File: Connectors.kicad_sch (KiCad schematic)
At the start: 13 parts, among them J5 Conn_02x03_Odd_Even, J6 Conn_02x03_Odd_Even, U12 TJA1051T/3

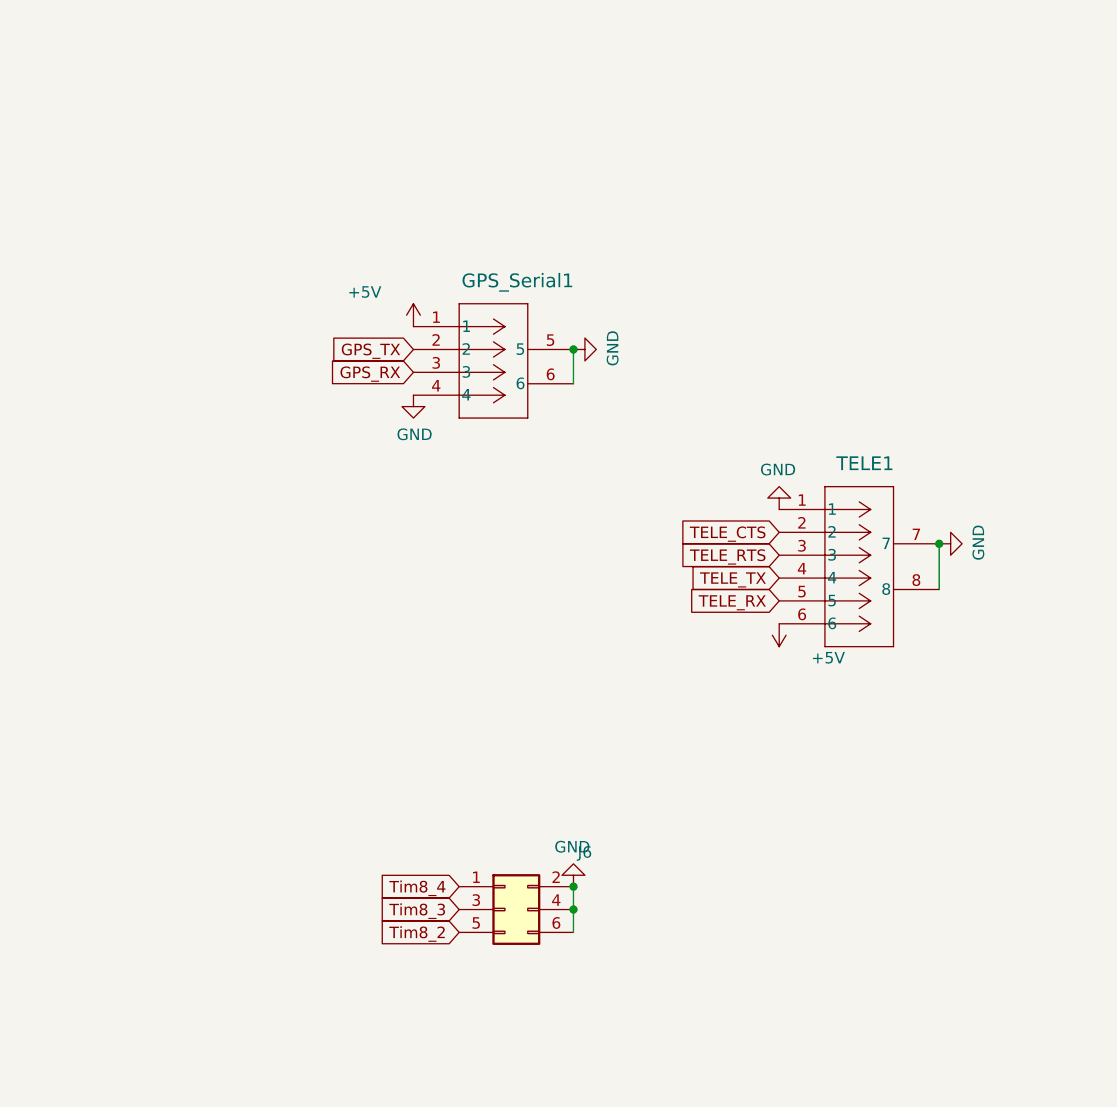
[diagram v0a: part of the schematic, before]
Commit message: PumbaaV2_RC2
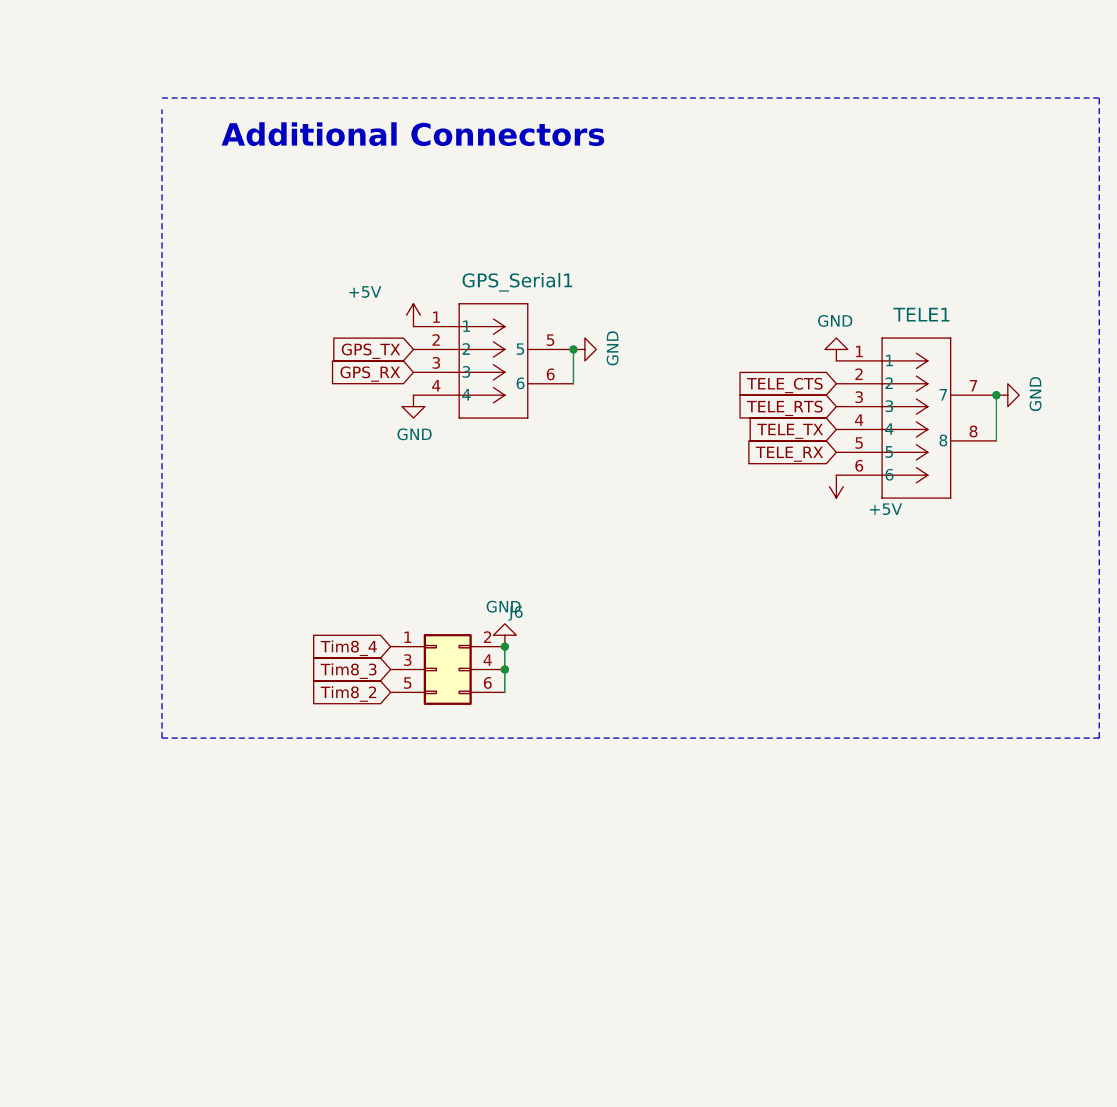
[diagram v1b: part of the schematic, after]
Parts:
- CAN1, GPS_Serial1: value SM04B-GHS-TB -> SM04B-GHS-TB(LF)(SN)
- R19: LCSC Part (none) -> C166918
- R20: LCSC (none) -> C166918
- TELE1: value SM06B-GHS-TB -> SM06B-GHS-TB(LF)(SN)
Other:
- note added: "Additional Connectors"
- moved on the sheet: J6, TELE1
